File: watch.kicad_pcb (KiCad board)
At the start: 2 copper layers, 34 x 34 mm, 72 parts, among them CON1 USB-MICRO-B, P1 CONN_6, SW1 SW_PUSH, SW2 SW_PUSH, SW3 SW_PUSH, SW4 SW_PUSH, U1 nrf51822, U2 ER-OLED015-1, U3 S25FL1-K, U4 74AHC1G14, U5 LTC4063, U6 FT230XQ, U7 TPS61093, U8 MMBD4148SE, X1 16MHz, X2 32.768kHz

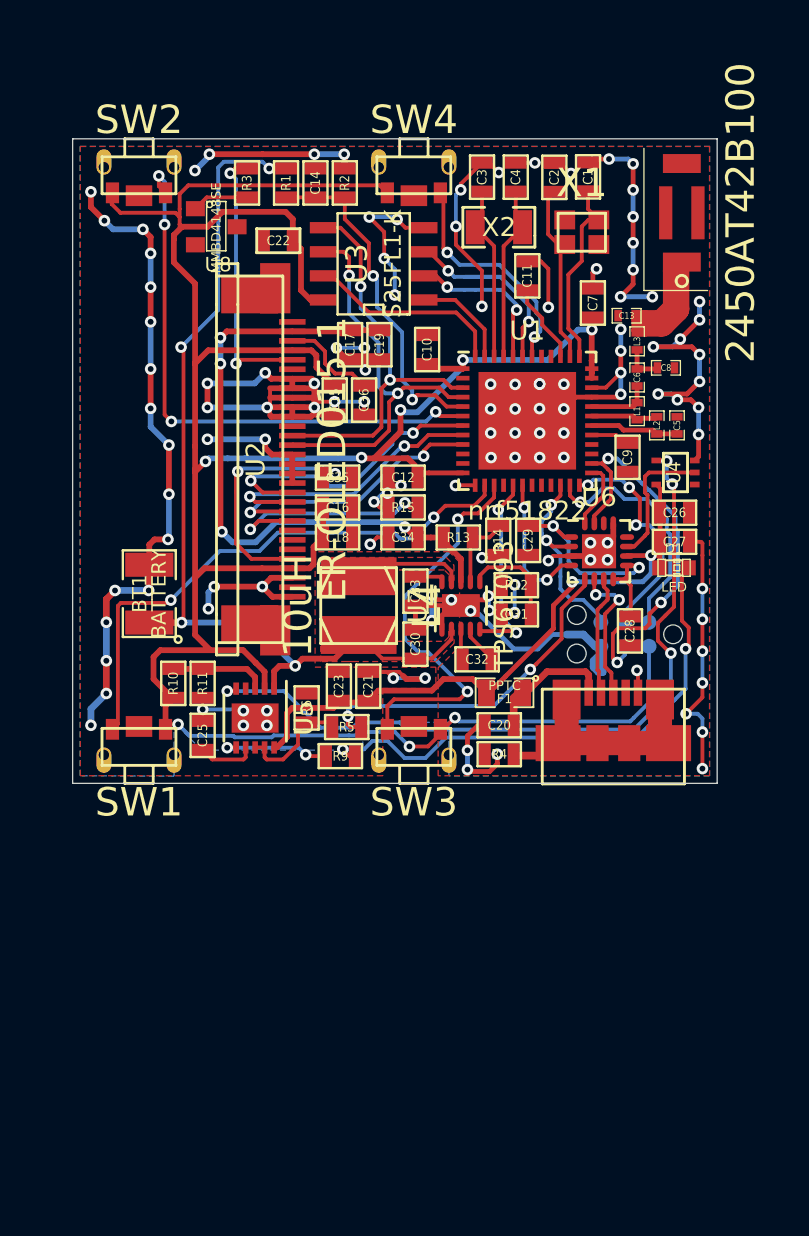
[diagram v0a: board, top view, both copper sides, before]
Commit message: Added .gitignore, finished midmount layout
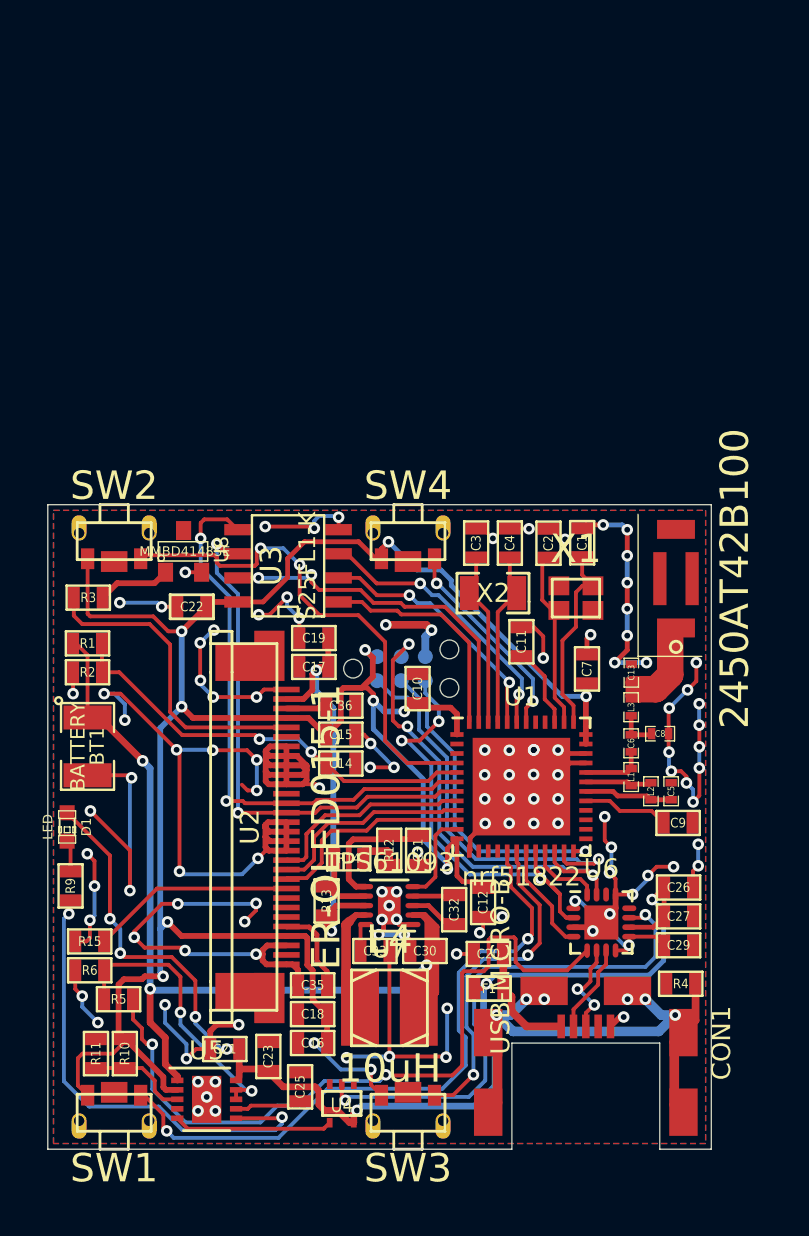
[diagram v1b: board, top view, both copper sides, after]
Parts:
- removed C28: 100nF, SMD_Packages:SMD-0603
- removed C34: 1uF, SMD_Packages:SMD-0603
- CON1: footprint Omat:USB_MICRO_AB_FEMALE -> Omat:USB_MICRO_B_FEMALE_MIDMOUNT
- F1: value PPTC -> MF-FSMF050X-2; footprint SMD_Packages:SMD-0805 -> SMD_Packages:SMD-0603
- P1: footprint TC2030-MCP-NL -> Omat:TC2030-MCP-NL
- moved U4 37.7 mm to (75.5, 91.6), turned to 270 degrees
- moved D1 34.8 mm to (61.0, 77.0), turned to 270 degrees
- moved C14 30.7 mm to (75.5, 73.7), turned to 180 degrees
- moved R2 29.2 mm to (62.1, 68.8), turned to 180 degrees
- moved C16 28.3 mm to (74.0, 88.4), turned to 180 degrees
- moved R15 28.2 mm to (62.2, 83.0)
- moved C35 26.8 mm to (74.0, 85.3), turned to 180 degrees
- moved R1 26.4 mm to (62.1, 67.3), turned to 0 degrees
- moved C18 25.2 mm to (74.0, 86.9), turned to 180 degrees
- moved R3 23.4 mm to (62.1, 64.9), turned to 0 degrees
- moved C12 22.8 mm to (83.0, 81.0), turned to 90 degrees
- moved C29 22.8 mm to (93.3, 83.2), turned to 0 degrees
- moved L4 21.3 mm to (78.0, 86.5), turned to 180 degrees
- moved C21 20.6 mm to (69.3, 88.7), turned to 180 degrees
- moved R13 20.4 mm to (74.7, 80.9), turned to 270 degrees
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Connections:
- ANT1 pad 2: Net-(ANT1-Pad2) -> (no net)
- ANT1 pad 3: Net-(ANT1-Pad3) -> (no net)
- ANT1 pad 4: Net-(ANT1-Pad4) -> (no net)
- CON1 pad 4: Net-(CON1-Pad4) -> (no net)
- SW1 pad 1: /SW1 -> +3.3V
- SW1 pad 2: +3.3V -> /SW1
- SW3 pad 1: /SW3 -> +3.3V
- SW3 pad 2: +3.3V -> /SW3
- U1 pad 10: Net-(U1-Pad10) -> CS_DISP
- U1 pad 11: Net-(U1-Pad11) -> DISP_EN
- U1 pad 14: /SW1 -> (no net)
- U1 pad 15: /SW3 -> (no net)
- U1 pad 16: Net-(U1-Pad16) -> (no net)
- U1 pad 17: DISP_EN -> /SW1
- U1 pad 18: MCU_RTS -> /SW3
- U1 pad 19: Net-(U1-Pad19) -> MCU_RTS
- U1 pad 2: Net-(U1-Pad2) -> (no net)
- U1 pad 20: Net-(U1-Pad20) -> MCU_TX
- U1 pad 21: Net-(U1-Pad21) -> MCU_CTS
- U1 pad 22: MCU_TX -> MCU_RX
- U1 pad 25: MCU_CTS -> (no net)
- U1 pad 26: MCU_RX -> (no net)
- U1 pad 27: Net-(U1-Pad27) -> (no net)
- U1 pad 28: Net-(U1-Pad28) -> (no net)
- U1 pad 3: MOSI -> (no net)
- U1 pad 4: SCK -> /SW2
- U1 pad 40: Net-(U1-Pad40) -> (no net)
- U1 pad 41: Net-(U1-Pad41) -> (no net)
- U1 pad 47: /CS_MEM -> /HOLD_MEM
- U1 pad 48: /HOLD_MEM -> /CS_MEM
- U1 pad 6: /SW2 -> MOSI
- U1 pad 7: RST_DISP -> SCK
- U1 pad 8: DC_DISP -> RST_DISP
- U1 pad 9: CS_DISP -> DC_DISP
- U2 pad 12: Net-(U2-Pad12) -> (no net)
- U2 pad 23: Net-(U2-Pad23) -> (no net)
- U2 pad 24: Net-(U2-Pad24) -> (no net)
- U2 pad 25: Net-(U2-Pad25) -> (no net)
- U2 pad 29: Net-(U2-Pad29) -> (no net)
- U2 pad 6: Net-(U2-Pad6) -> (no net)
- U5 pad 4: Net-(U5-Pad4) -> (no net)
- U6 pad 12: Net-(U6-Pad12) -> (no net)
- U6 pad 14: Net-(U6-Pad14) -> (no net)
- U8 pad 3: Net-(U8-Pad3) -> (no net)
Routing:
- net Net-(U4-Pad4): track 39.4 -> 8.40 mm, vias 4 -> 0
- net Net-(D1-Pad2): track 27.8 -> 1.67 mm, vias 2 -> 0
- net /watch_usb_power/VBUS: track 35.5 -> 61.5 mm, vias 2 -> 7
- net /watch_usb_power/~SLEEP: track 7.14 -> 27.7 mm, vias 0 -> 2
- net /watch_usb_power/~PWREN: track 18.5 -> 38.9 mm
- net Net-(R9-Pad1): track 5.87 -> 25.2 mm
- net +3.3V: track 152.4 -> 133.4 mm, vias 8 -> 12
- net MCU_TX: track 10.7 -> 23.3 mm, vias 2 -> 3
- net 12.5V: track 34.3 -> 22.6 mm, vias 4 -> 2
- net Net-(CON1-Pad6): track 20.3 -> 30.6 mm, vias 0 -> 6
- net Net-(R5-Pad2): track 6.04 -> 15.0 mm, vias 0 -> 2
- net Net-(C35-Pad1): track 13.4 -> 4.68 mm, vias 2 -> 0
- net MOSI: track 21.7 -> 30.3 mm
- net /HOLD_MEM: track 10.6 -> 18.8 mm, vias 0 -> 2
- net /SWDIO: track 13.2 -> 21.1 mm
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- removed copper zone on F.Cu, net /watch_usb_power/BOOST_SWITCH
- removed copper zone on F.Cu, net VBAT
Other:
- board size 34 x 34 mm -> 35 x 34 mm
